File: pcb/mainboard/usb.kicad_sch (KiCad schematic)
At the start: 73 parts

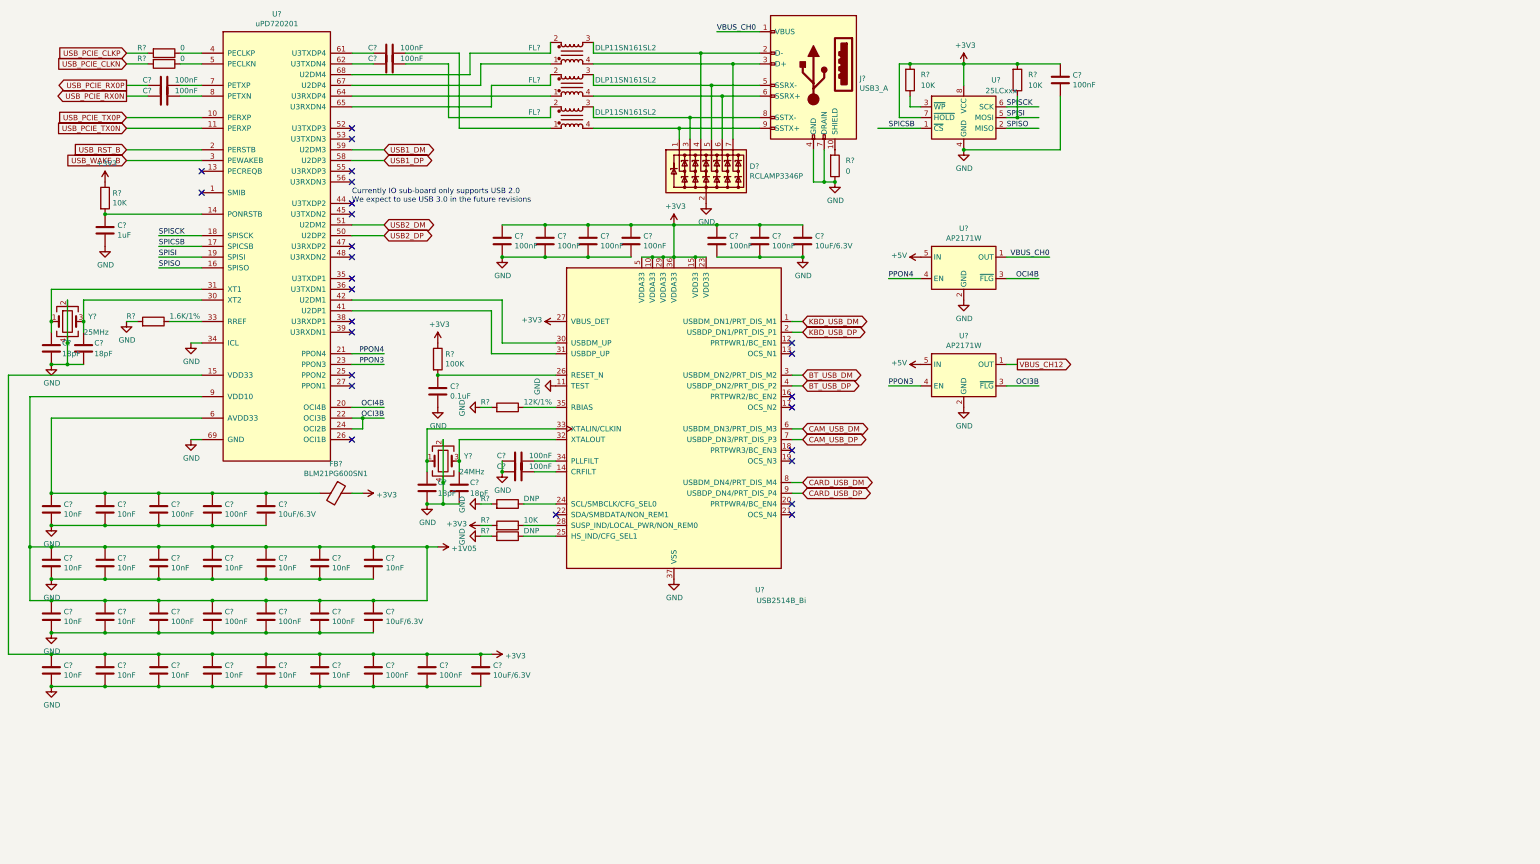
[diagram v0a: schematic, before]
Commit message: - Upgrade KiCad to latest version - Working on PM circuits - Initial USB Type-C support - Initial support for LCD
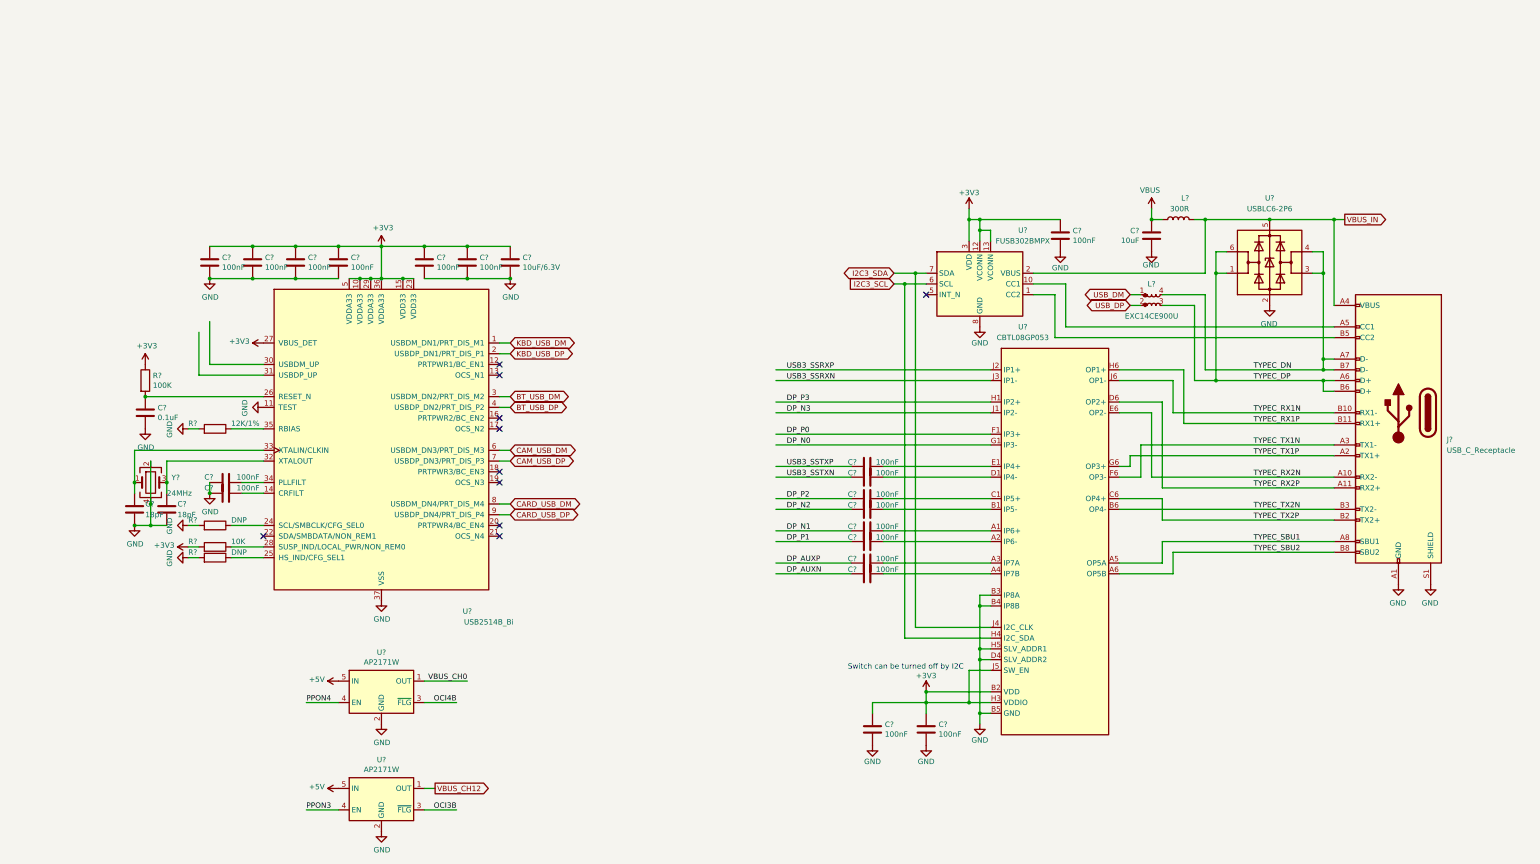
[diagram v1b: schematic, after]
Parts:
- removed C? (x2): 18pF, Capacitor_SMD:C_0603_1608Metric, symbol Device:C
- removed C? (x4): 100nF, Capacitor_SMD:C_0603_1608Metric, symbol Device:C
- removed C?: 1uF, symbol Device:C
- removed C? (x17): 10nF, symbol Device:C
- removed C? (x9): 100nF, symbol Device:C
- removed C? (x3): 10uF/6.3V, symbol Device:C
- removed D?: RCLAMP3346P, footprints:UDFN-7_0.8x2.7mm_P0.4mm, symbol symbols:RCLAMP3346P
- removed FB?: BLM21PG600SN1, symbol Device:Ferrite_Bead
- removed FL? (x3): DLP11SN161SL2, footprints:Filter_125100, symbol Device:EMI_Filter_LL_1423
- removed J?: USB3_A, footprints:USB3_A_1.36_SINK, symbol Connector:USB3_A
- removed R? (x3): 0, Resistor_SMD:R_0603_1608Metric, symbol Device:R
- removed R?: 1.6K/1%, Resistor_SMD:R_0603_1608Metric, symbol Device:R
- removed R?: 10K, symbol Device:R
- removed R? (x2): 10K, Resistor_SMD:R_0603_1608Metric, symbol Device:R
- removed U?: uPD720201, Package_DFN_QFN:QFN-68-1EP_8x8mm_P0.4mm_EP5.2x5.2mm_ThermalVias, symbol symbols:uPD720201
- removed U?: 25LCxxx, symbol Memory_EEPROM:25LCxxx
- removed Y?: 25MHz, Crystal:Crystal_SMD_3225-4Pin_3.2x2.5mm, symbol Device:Crystal_GND24
- added C? (x11): 100nF, Capacitor_SMD:C_0201_0603Metric, symbol Device:C
- added C?: 10uF, Capacitor_SMD:C_0402_1005Metric, symbol Device:C
- added J?: USB_C_Receptacle, Connector_USB:USB_C_Receptacle_Amphenol_12401548E4-2A, symbol Connector:USB_C_Receptacle
- added L?: EXC14CE900U, footprint:L_CommonModeChoke_Panasonic_EXC14CE, symbol Device:L_Coupled_Small_1423
- added L?: 300R, Inductor_SMD:L_0603_1608Metric, symbol Device:L
- added U?: USBLC6-2P6, Package_TO_SOT_SMD:SOT-666, symbol Power_Protection:USBLC6-2P6
- added U?: CBTL08GP053, footprint:BGA-40_6x9_3.5x5.0mm, symbol symbols:CBTL08GP053
- added U?: FUSB302BMPX, Package_DFN_QFN:WQFN-14-1EP_2.5x2.5mm_P0.5mm_EP1.45x1.45mm, symbol Interface_USB:FUSB302BMPX
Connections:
- net +3V3: now also C?.1, C?.1, C?.1, U?.12 (VCONN), U?.13 (VCONN), U?.3 (VDD), U?.4 (VDD), U?.B2 (VDD), U?.E3 (VDD), U?.E4 (VDDIO), U?.H3 (VDDIO), U?.J5 (SW_EN)
- net GND: now also C?.2, C?.2, C?.2, C?.2, J?.A1 (GND), J?.A12 (GND), J?.B1 (GND), J?.B12 (GND), J?.S1 (SHIELD), U?.15 (GND), U?.2 (GND), U?.8 (GND), U?.9 (GND), U?.B3 (IP8A), U?.B4 (IP8B), U?.B5 (GND), U?.D3 (GND), U?.D4 (SLV_ADDR2), U?.F3 (GND), U?.F4 (GND), U?.H2 (GND), U?.H5 (SLV_ADDR1)
- new net: C?.2, U?.A1 (IP6+)
- new net: C?.2, U?.B1 (IP5-)
- new net: C?.2, U?.A2 (IP6-)
- new net: C?.2, U?.A4 (IP7B)
- new net: C?.2, U?.C1 (IP5+)
- new net: J?.A5 (CC1), U?.10 (CC1), U?.11 (CC1)
- new net: J?.B5 (CC2), U?.1 (CC2), U?.14 (CC2)
- new net: C?.2, U?.A3 (IP7A)
- new net: C?.2, U?.D1 (IP4-)
- new net: C?.2, U?.E1 (IP4+)
- new net DP_AUXN: C?.1
- new net DP_AUXP: C?.1
- new net DP_N0: U?.G1 (IP3-)
- new net DP_N1: C?.1
- new net DP_N2: C?.1
- new net DP_N3: U?.J1 (IP2-)
- new net DP_P0: U?.F1 (IP3+)
- new net DP_P1: C?.1
- new net DP_P2: C?.1
- new net DP_P3: U?.H1 (IP2+)
- new net I2C3_SCL: U?.6 (SCL), U?.H4 (I2C_SDA)
- new net I2C3_SDA: U?.7 (SDA), U?.J4 (I2C_CLK)
- new net TYPEC_DN: J?.A7 (D-), J?.B7 (D-), L?.4, U?.3 (I/O2), U?.4 (I/O2)
- new net TYPEC_DP: J?.A6 (D+), J?.B6 (D+), L?.3, U?.1 (I/O1), U?.6 (I/O1)
- new net TYPEC_RX1N: J?.B10 (RX1-), U?.J6 (OP1-)
- new net TYPEC_RX1P: J?.B11 (RX1+), U?.H6 (OP1+)
- new net TYPEC_RX2N: J?.A10 (RX2-), U?.E6 (OP2-)
- new net TYPEC_RX2P: J?.A11 (RX2+), U?.D6 (OP2+)
- new net TYPEC_SBU1: J?.A8 (SBU1), U?.A5 (OP5A)
- new net TYPEC_SBU2: J?.B8 (SBU2), U?.A6 (OP5B)
- new net TYPEC_TX1N: J?.A3 (TX1-), U?.F6 (OP3-)
- new net TYPEC_TX1P: J?.A2 (TX1+), U?.G6 (OP3+)
- new net TYPEC_TX2N: J?.B3 (TX2-), U?.B6 (OP4-)
- new net TYPEC_TX2P: J?.B2 (TX2+), U?.C6 (OP4+)
- new net USB3_SSRXN: U?.J3 (IP1-)
- new net USB3_SSRXP: U?.J2 (IP1+)
- new net USB3_SSTXN: C?.1
- new net USB3_SSTXP: C?.1
- new net USB_DM: L?.1
- new net USB_DP: L?.2
- new net VBUS: C?.1, L?.1
- new net VBUS_IN: J?.A4 (VBUS), J?.A9 (VBUS), J?.B4 (VBUS), J?.B9 (VBUS), L?.2, U?.2 (VBUS), U?.5 (VBUS)
- no-connect marks 26 -> 10
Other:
- note added: "Switch can be turned off by I2C"
- note removed: "Currently IO sub-board only supports USB 2.0 We expect to use USB 3.0 in the future revisions"
- moved on the sheet: C?, R?, U?, Y?
